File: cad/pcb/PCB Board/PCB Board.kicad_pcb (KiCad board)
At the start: 2 copper layers, 70 x 70 mm, 10 parts, among them J1 POWER, J2 LED+, J3 Conn_01x02_Pin, SW1 SW_Push, SW2 SW_Push, SW3 SW_Push, SW4 SW_Push, U1 BOB-12009

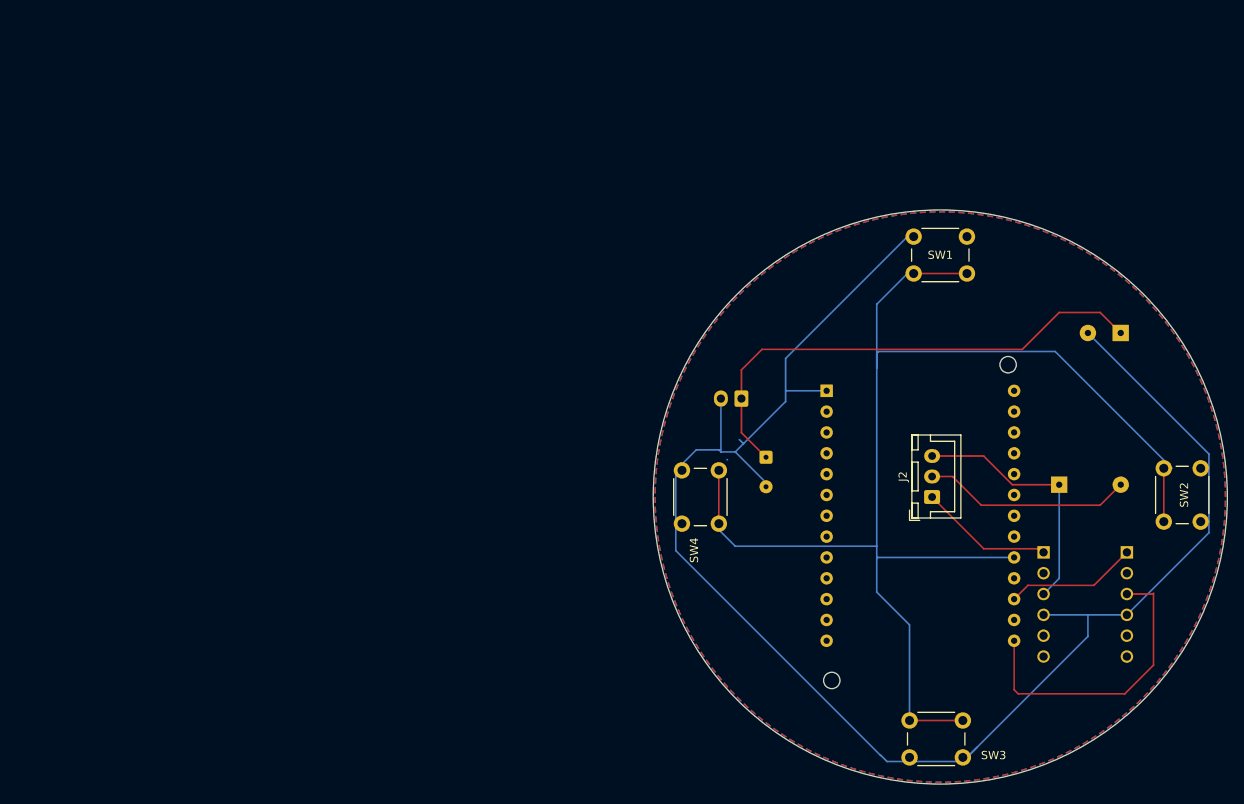
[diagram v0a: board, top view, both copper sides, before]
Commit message: updated pcbs
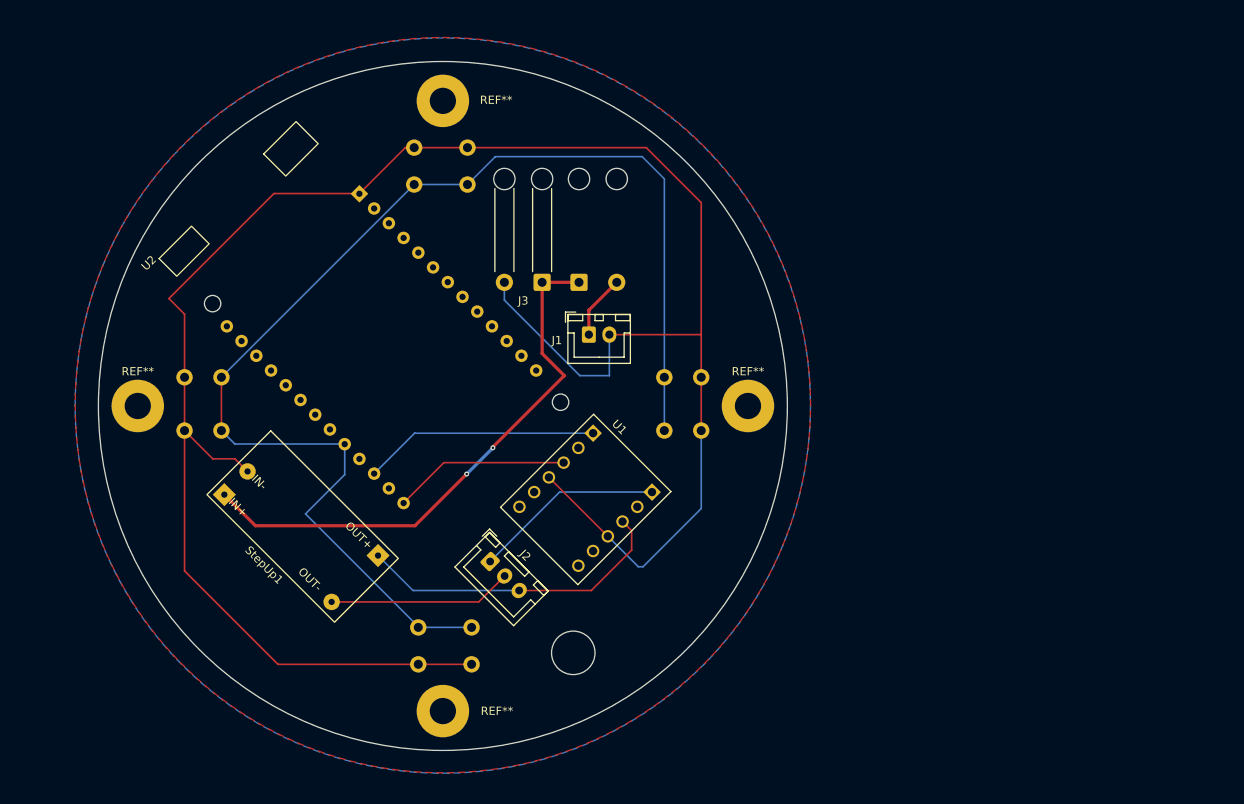
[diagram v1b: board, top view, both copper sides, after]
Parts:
- added J4: ON_OFF_SWITCH, Connector_Wire:SolderWire-0.5sqmm_1x02_P4.6mm_D0.9mm_OD2.1mm_Relief, B.Cu at (81.2, 48.8)
- added REF**: MountingHole_3.2mm_M3_Pad, MountingHole:MountingHole_3.2mm_M3_Pad, F.Cu at (101.8, 63.9)
- added REF**: MountingHole_3.2mm_M3_Pad, MountingHole:MountingHole_3.2mm_M3_Pad, F.Cu at (64.6, 101.1)
- added REF**: MountingHole_5.3mm_M5_DIN965, MountingHole:MountingHole_5.3mm_M5_DIN965, F.Cu at (80.5, 94.0)
- added REF**: MountingHole_3.2mm_M3_Pad, MountingHole:MountingHole_3.2mm_M3_Pad, F.Cu at (27.4, 63.9)
- added REF**: MountingHole_3.2mm_M3_Pad, MountingHole:MountingHole_3.2mm_M3_Pad, F.Cu at (64.6, 26.7)
- J1, StepUp1, U2: moved to F.Cu
- J3: value Conn_01x02_Pin -> BATTERY_CONNECTOR; footprint Connector_Wire:SolderWire-0.1sqmm_1x02_P3.6mm_D0.4mm_OD1mm -> Connector_Wire:SolderWire-0.5sqmm_1x02_P4.6mm_D0.9mm_OD2.1mm_Relief; moved to F.Cu
- SW1, SW2, SW3, SW4: moved to B.Cu
- U1: value BOB-12009 -> Lvl-Shifter; moved to F.Cu
- moved SW2 124.4 mm to (33.1, 60.4)
- moved U2 106.5 mm to (29.1, 46.8), turned to 45 degrees
- moved StepUp1 96.8 mm to (47.5, 78.6), turned to -45 degrees
- moved SW3 67.4 mm to (61.6, 95.4), turned to 0 degrees
- moved U1 62.2 mm to (82.0, 75.3), turned to -45 degrees
- moved SW1 55.5 mm to (67.6, 32.4), turned to 180 degrees
- moved J2 54.5 mm to (70.4, 82.9), turned to -45 degrees
- moved J3 34.6 mm to (76.7, 48.8), turned to 180 degrees
- moved J1 20.2 mm to (82.4, 55.2), turned to 0 degrees
- moved SW4 11.6 mm to (96.1, 66.9)
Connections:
- J1 pad 2: GND -> Net-(J1-Pin_2)
- J3 pad 1: Net-(J1-Pin_1) -> Net-(J3-Pin_1)
- J3 pad 2: GND -> Net-(J1-Pin_2)
- SW2 pad 1: GND -> Net-(J1-Pin_2)
- SW3 pad 1: GND -> Net-(J1-Pin_2)
- SW4 pad 1: GND -> Net-(J1-Pin_2)
- StepUp1 pad 1: GND -> Net-(J1-Pin_2)
- StepUp1 pad 2: Net-(J1-Pin_1) -> Net-(J3-Pin_1)
- U1 pad GND_1: GND -> Net-(J1-Pin_2)
- U1 pad GND_2: GND -> Net-(J1-Pin_2)
- U2 pad GND: GND -> Net-(J1-Pin_2)
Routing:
- net Net-(J1-Pin_2): track 0.00 -> 257.2 mm
- net GND: track 199.4 -> 0.00 mm
- net Net-(J3-Pin_1): track 0.00 -> 67.7 mm, vias 0 -> 2
- net Net-(J1-Pin_1): track 62.1 -> 7.78 mm
- net Net-(U1-PadLV): track 36.7 -> 21.5 mm
- net Net-(U1-PadLV1): track 16.1 -> 28.7 mm
- net Net-(SW1-Pad2): track 167.0 -> 155.8 mm
- net Net-(J2-Pin_3): track 31.1 -> 38.7 mm
- net Net-(J2-Pin_1): track 16.4 -> 23.2 mm
- net Net-(J2-Pin_2): track 25.5 -> 22.4 mm
- added copper zone on B.Cu, net Net-(J1-Pin_2)
- added copper zone on F.Cu, net Net-(J1-Pin_2)
- removed copper zone on B.Cu, net GND
- removed copper zone on F.Cu, net GND
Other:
- board size 70 x 70 mm -> 84 x 84 mm

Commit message: [WIP] save changes
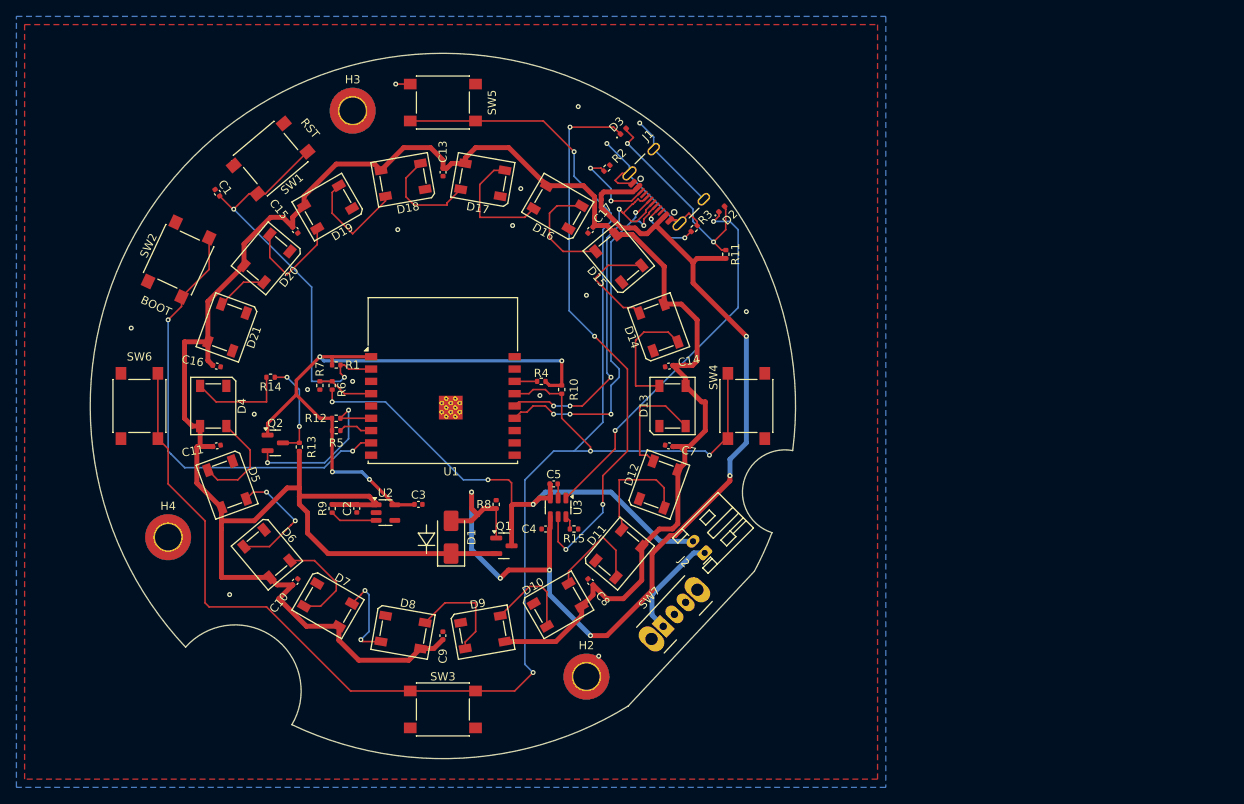
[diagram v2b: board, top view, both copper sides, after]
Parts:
- removed J3: BATTERY_CONNECTOR, Connector_Wire:SolderWire-0.5sqmm_1x02_P4.6mm_D0.9mm_OD2.1mm_Relief
- removed J4: ON_OFF_SWITCH, Connector_Wire:SolderWire-0.5sqmm_1x02_P4.6mm_D0.9mm_OD2.1mm_Relief
- removed REF** (x4): MountingHole_3.2mm_M3_Pad, MountingHole:MountingHole_3.2mm_M3_Pad
- removed REF**: MountingHole_5.3mm_M5_DIN965, MountingHole:MountingHole_5.3mm_M5_DIN965
- removed StepUp1: ~, Library:StepUp
- added C1: C1uF, Capacitor_SMD:C_0402_1005Metric, F.Cu at (37.1, 37.9)
- added C10: C1uF, Capacitor_SMD:C_0402_1005Metric, F.Cu at (46.6, 85.3)
- added C11: C1uF, Capacitor_SMD:C_0402_1005Metric, F.Cu at (37.0, 68.8)
- added C13: C1uF, Capacitor_SMD:C_0402_1005Metric, F.Cu at (64.6, 35.4)
- added C14: C1uF, Capacitor_SMD:C_0402_1005Metric, F.Cu at (92.2, 59.0)
- added C15: C1uF, Capacitor_SMD:C_0402_1005Metric, F.Cu at (46.6, 42.5)
- added C16: C1uF, Capacitor_SMD:C_0402_1005Metric, F.Cu at (37.0, 59.0)
- added C17: C1uF, Capacitor_SMD:C_0402_1005Metric, F.Cu at (82.6, 42.5)
- added C2: C10uF, Capacitor_SMD:C_0402_1005Metric, F.Cu at (54.1, 76.4)
- added C3: C1uF, Capacitor_SMD:C_0402_1005Metric, F.Cu at (61.6, 75.9)
- added C4: C2.2uF, Capacitor_SMD:C_0402_1005Metric, F.Cu at (77.1, 78.9)
- added C5: C10uF, Capacitor_SMD:C_0402_1005Metric, F.Cu at (78.1, 73.4)
- added C7: C1uF, Capacitor_SMD:C_0402_1005Metric, F.Cu at (92.2, 68.8)
- added C8: C1uF, Capacitor_SMD:C_0402_1005Metric, F.Cu at (82.6, 85.3)
- added C9: C1uF, Capacitor_SMD:C_0402_1005Metric, F.Cu at (64.6, 91.9)
- added D1: SS14, Diode_SMD:D_SMA, F.Cu at (65.6, 79.9)
- added D10: SK6812, LED_SMD:LED_SK6812_PLCC4_5.0x5.0mm_P3.2mm, F.Cu at (78.6, 88.1)
- added D11: SK6812, LED_SMD:LED_SK6812_PLCC4_5.0x5.0mm_P3.2mm, F.Cu at (86.0, 81.9)
- added D12: SK6812, LED_SMD:LED_SK6812_PLCC4_5.0x5.0mm_P3.2mm, F.Cu at (90.9, 73.5)
- added D13: SK6812, LED_SMD:LED_SK6812_PLCC4_5.0x5.0mm_P3.2mm, F.Cu at (92.6, 63.9)
- added D14: SK6812, LED_SMD:LED_SK6812_PLCC4_5.0x5.0mm_P3.2mm, F.Cu at (90.9, 54.3)
- added D15: SK6812, LED_SMD:LED_SK6812_PLCC4_5.0x5.0mm_P3.2mm, F.Cu at (86.0, 45.9)
- added D16: SK6812, LED_SMD:LED_SK6812_PLCC4_5.0x5.0mm_P3.2mm, F.Cu at (78.6, 39.7)
- added D17: SK6812, LED_SMD:LED_SK6812_PLCC4_5.0x5.0mm_P3.2mm, F.Cu at (69.5, 36.3)
- added D18: SK6812, LED_SMD:LED_SK6812_PLCC4_5.0x5.0mm_P3.2mm, F.Cu at (59.7, 36.3)
- added D19: SK6812, LED_SMD:LED_SK6812_PLCC4_5.0x5.0mm_P3.2mm, F.Cu at (50.6, 39.7)
- added D2: 150040VS73220, LED_SMD:LED_0402_1005Metric, F.Cu at (98.6, 39.9)
- added D20: SK6812, LED_SMD:LED_SK6812_PLCC4_5.0x5.0mm_P3.2mm, F.Cu at (43.2, 45.9)
- added D21: SK6812, LED_SMD:LED_SK6812_PLCC4_5.0x5.0mm_P3.2mm, F.Cu at (38.3, 54.3)
- added D3: 150040BS73220, LED_SMD:LED_0402_1005Metric, F.Cu at (86.6, 30.4)
- added D4: SK6812, LED_SMD:LED_SK6812_PLCC4_5.0x5.0mm_P3.2mm, F.Cu at (36.6, 63.9)
- added D5: SK6812, LED_SMD:LED_SK6812_PLCC4_5.0x5.0mm_P3.2mm, F.Cu at (38.3, 73.5)
- added D6: SK6812, LED_SMD:LED_SK6812_PLCC4_5.0x5.0mm_P3.2mm, F.Cu at (43.2, 81.9)
- added D7: SK6812, LED_SMD:LED_SK6812_PLCC4_5.0x5.0mm_P3.2mm, F.Cu at (50.6, 88.1)
- added D8: SK6812, LED_SMD:LED_SK6812_PLCC4_5.0x5.0mm_P3.2mm, F.Cu at (59.7, 91.5)
- added D9: SK6812, LED_SMD:LED_SK6812_PLCC4_5.0x5.0mm_P3.2mm, F.Cu at (69.5, 91.5)
- added H2: MountingHole_Pad, MountingHole:MountingHole_3.2mm_M3_DIN965_Pad_TopBottom, F.Cu at (82.1, 96.9)
- added H3: MountingHole_Pad, MountingHole:MountingHole_3.2mm_M3_DIN965_Pad_TopBottom, F.Cu at (53.6, 27.9)
- added H4: MountingHole_Pad, MountingHole:MountingHole_3.2mm_M3_DIN965_Pad_TopBottom, F.Cu at (31.1, 79.9)
- added Q1: FDN340P, Package_TO_SOT_SMD:SOT-23, F.Cu at (72.0, 81.0)
- added Q2: BSS138, Package_TO_SOT_SMD:SOT-23, F.Cu at (44.2, 68.4)
- added R1: R10K, Resistor_SMD:R_0402_1005Metric, F.Cu at (51.6, 58.9)
- added R10: R10K, Resistor_SMD:R_0402_1005Metric, F.Cu at (79.1, 61.9)
- added R11: R330, Resistor_SMD:R_0402_1005Metric, F.Cu at (99.1, 45.4)
- added R12: R10K, Resistor_SMD:R_0402_1005Metric, F.Cu at (51.6, 65.4)
- added R13: R10K, Resistor_SMD:R_0402_1005Metric, F.Cu at (47.1, 68.9)
- added R14: R470, Resistor_SMD:R_0402_1005Metric, F.Cu at (43.6, 60.4)
- added R15: R2K, Resistor_SMD:R_0402_1005Metric, F.Cu at (80.6, 78.9)
- added R2: R5.1k, Resistor_SMD:R_0402_1005Metric, F.Cu at (84.6, 34.9)
- added R3: R5.1k, Resistor_SMD:R_0402_1005Metric, F.Cu at (95.2, 42.3)
- added R4: R10K, Resistor_SMD:R_0402_1005Metric, F.Cu at (76.6, 60.9)
- added R5: R10K, Resistor_SMD:R_0402_1005Metric, F.Cu at (51.6, 66.9)
- added R6: R100K, Resistor_SMD:R_0402_1005Metric, F.Cu at (51.1, 61.4)
- added R7: R100K, Resistor_SMD:R_0402_1005Metric, F.Cu at (49.6, 61.4)
- added R8: R100K, Resistor_SMD:R_0402_1005Metric, F.Cu at (71.1, 75.9)
- added R9: R100K, Resistor_SMD:R_0402_1005Metric, F.Cu at (51.1, 76.4)
- added SW5: PTS645, Button_Switch_SMD:SW_SPST_PTS645, F.Cu at (64.6, 26.9)
- added SW6: PTS645, Button_Switch_SMD:SW_SPST_PTS645, F.Cu at (27.6, 63.9)
- added SW7: SLW-1277545-3A-RA-N-D, Button_Switch_THT:SW_Slide_SPDT_Angled_CK_OS102011MA1Q, F.Cu at (91.5, 90.8)
- added U3: TP4057, Package_TO_SOT_SMD:TSOT-23-6, F.Cu at (78.7, 76.3)
- J1: value POWER -> USB4105; footprint Connector_JST:JST_XH_B2B-XH-A_1x02_P2.50mm_Vertical -> Connector_USB:USB_C_Receptacle_GCT_USB4105-xx-A_16P_TopMnt_Horizontal
- J2: value LED+ -> S2B-PH-K-S; footprint Connector_JST:JST_XH_B3B-XH-A_1x03_P2.50mm_Vertical -> Connector_JST:JST_PH_S2B-PH-K_1x02_P2.00mm_Horizontal
- SW1, SW2, SW3, SW4: value SW_Push -> PTS645; footprint Button_Switch_THT:SW_PUSH_6mm_H5mm -> Button_Switch_SMD:SW_SPST_PTS645; moved to F.Cu
- U1: value Lvl-Shifter -> ESP32-C3-WROOM-02; footprint BOB-12009:CONV_BOB-12009 -> RF_Module:ESP32-C3-WROOM-02
- U2: value ~ -> TLV75533PDYDR; footprint Library:Lolin32 Lite -> Package_TO_SOT_SMD:SOT-23-5
- moved U2 41.4 mm to (57.6, 76.9), turned to 0 degrees
- moved J2 26.2 mm to (96.5, 81.8), turned to 135 degrees
- moved SW1 24.0 mm to (43.6, 33.7), turned to -140 degrees
- moved J1 21.4 mm to (92.6, 36.4), turned to 135 degrees
- moved U1 20.8 mm to (64.6, 63.9), turned to 0 degrees
- moved SW2 14.4 mm to (32.4, 46.1), turned to 65 degrees
- moved SW4 6.26 mm to (101.6, 63.9), turned to -90 degrees
- moved SW3 6.26 mm to (64.6, 100.9), turned to 180 degrees
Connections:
- J2 pad 2: Net-(J2-Pin_2) -> VBAT
- SW1 pad 1: Net-(J1-Pin_2) -> EN
- SW1 pad 2: Net-(SW1-Pad2) -> GND
- SW2 pad 1: Net-(J1-Pin_2) -> GND
- SW2 pad 2: Net-(SW1-Pad2) -> IO9
- SW3 pad 1: Net-(J1-Pin_2) -> GND
- SW3 pad 2: Net-(SW1-Pad2) -> IO3
- SW4 pad 1: Net-(J1-Pin_2) -> GND
- SW4 pad 2: Net-(SW1-Pad2) -> IO3
- U2 pad 2: unconnected-(U2-Pad2) -> GND
- U2 pad 5: unconnected-(U2-Pad5) -> 3V3
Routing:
- net VIN: track 0.00 -> 297.9 mm
- net Net-(J1-Pin_2): track 257.2 -> 0.00 mm
- net IO3: track 0.00 -> 211.2 mm, vias 0 -> 4
- net Net-(SW1-Pad2): track 155.8 -> 0.00 mm
- net VBUS: track 0.00 -> 133.0 mm, vias 0 -> 6
- net 3V3: track 0.00 -> 78.1 mm, vias 0 -> 4
- net Net-(D3-K): track 0.00 -> 68.5 mm, vias 0 -> 4
- net Net-(J3-Pin_1): track 67.7 -> 0.00 mm, vias 2 -> 0
- net VBAT: track 0.00 -> 64.6 mm, vias 0 -> 3
- net IO9: track 0.00 -> 54.9 mm, vias 0 -> 2
- net EN: track 0.00 -> 49.1 mm, vias 0 -> 2
- net D-: track 0.00 -> 46.5 mm, vias 0 -> 5
- net Net-(D2-K): track 0.00 -> 46.3 mm, vias 0 -> 2
- net D+: track 0.00 -> 45.3 mm, vias 0 -> 4
- net GND: track 0.00 -> 40.6 mm, vias 0 -> 16
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- added copper zone on B.Cu, net GND
- added copper zone on F.Cu, net GND
- removed copper zone on B.Cu, net Net-(J1-Pin_2)
- removed copper zone on F.Cu, net Net-(J1-Pin_2)
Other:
- board size 84 x 84 mm -> 86 x 86 mm
- board text added: "BOOT"
- board text added: "RST"
